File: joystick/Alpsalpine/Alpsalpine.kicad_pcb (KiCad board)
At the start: 2 copper layers, 26 x 26 mm, 6 parts

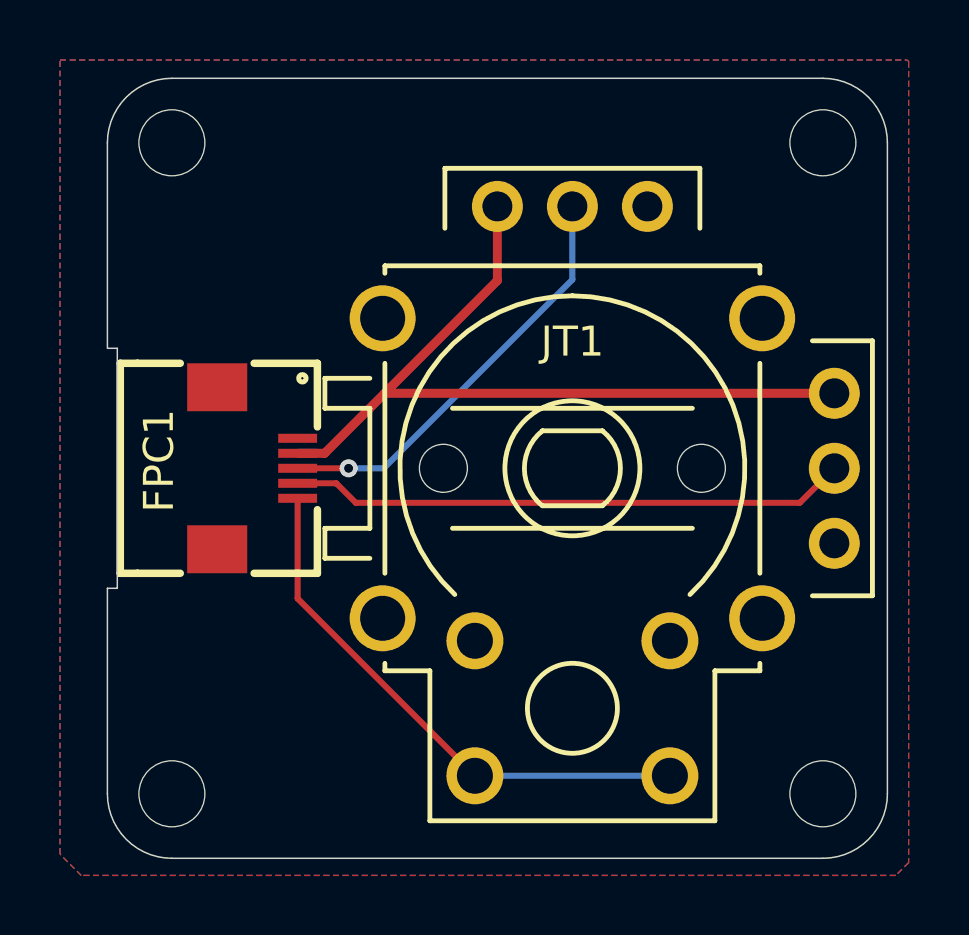
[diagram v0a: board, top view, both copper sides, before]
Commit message: update joystick mount
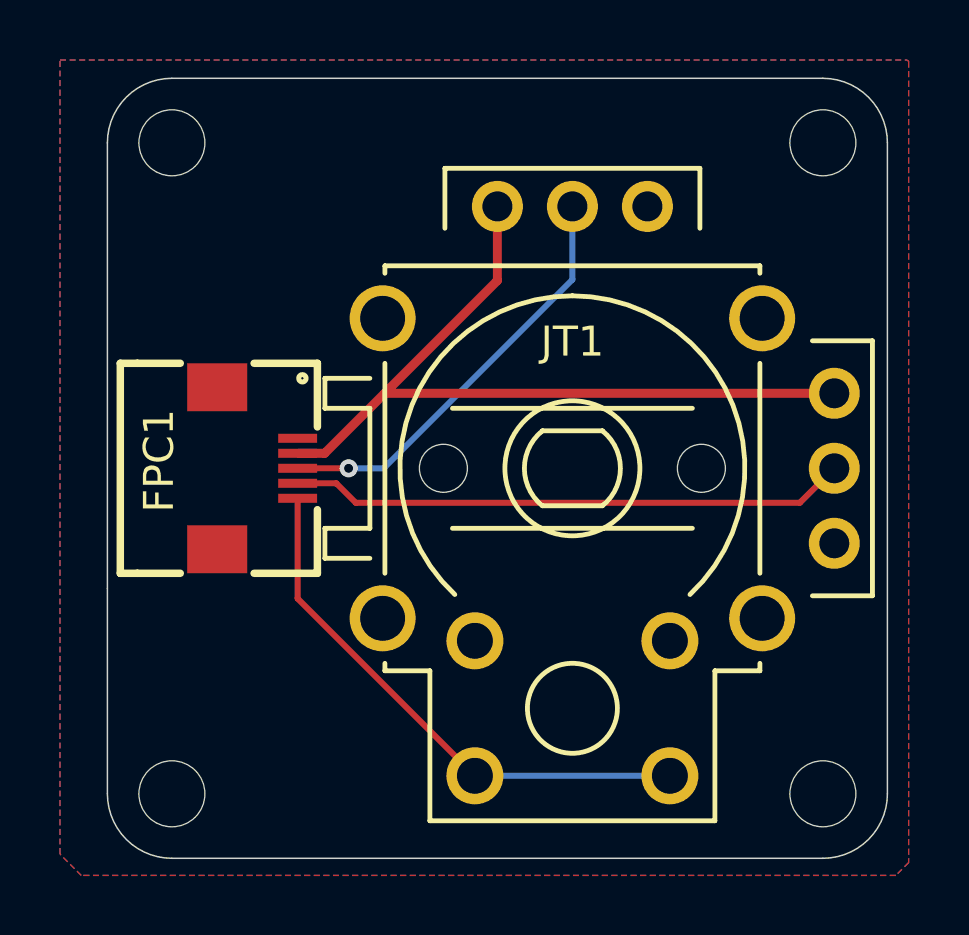
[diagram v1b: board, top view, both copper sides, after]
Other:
- outline, holes or cut-outs redrawn
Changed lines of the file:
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@@
 		)
 		(embedded_fonts no)
-		(model "${EASYEDA2KICAD}/easyeda2kicad.3dshapes/FPC-SMD_AFC01-S05FCA-00.wrl"
-			(offset
-				(xyz 0 -1.32 -0)
-			)
-			(scale
-				(xyz 1 1 1)
-			)
-			(rotate
-				(xyz 0 0 0)
-			)
-		)
-		(model "/Users/jinsongc/Documents/KiCad/easyeda2kicad/easyeda2kicad.3dshapes/FPC-SMD_AFC01-S05FCA-00.step"
+		(model "/Users/jinsongc/Development/ErgoCaiLib/3dmodels/FPC-SMD_AFC01-S05FCA-00.step"
 			(offset
 				(xyz 0 -1 2)
@@
 	)
 	(gr_line
-		(start -12.67 -4)
-		(end -12.67 4)
-		(stroke
-			(width 0.05)
-			(type solid)
-		)
-		(layer "Edge.Cuts")
-	)
-	(gr_line
 		(start 13 10.85)
 		(end 13 -10.85)
@@
 		(layer "Edge.Cuts")
 	)
-	(gr_line
-		(start -12.99 -4)
-		(end -12.67 -4)
-		(stroke
-			(width 0.05)
-			(type solid)
-		)
-		(layer "Edge.Cuts")
-	)
 	(gr_arc
 		(start 13 10.85)
 		(mid 12.37028 12.37028)
 		(end 10.85 13)
-		(stroke
-			(width 0.05)
-			(type solid)
-		)
-		(layer "Edge.Cuts")
-	)
-	(gr_line
-		(start -12.67 4)
-		(end -13 4)
 		(stroke
 			(width 0.05)
@@
 	(gr_line
 		(start -12.999999 -10.85)
-		(end -12.999999 -4)
+		(end -12.999999 4)
 		(stroke
 			(width 0.05)
